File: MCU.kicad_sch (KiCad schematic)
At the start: 18 parts, among them U1 STM32L476RCTx, U3 LD1117S33TR, U5 nRF2401+ Module

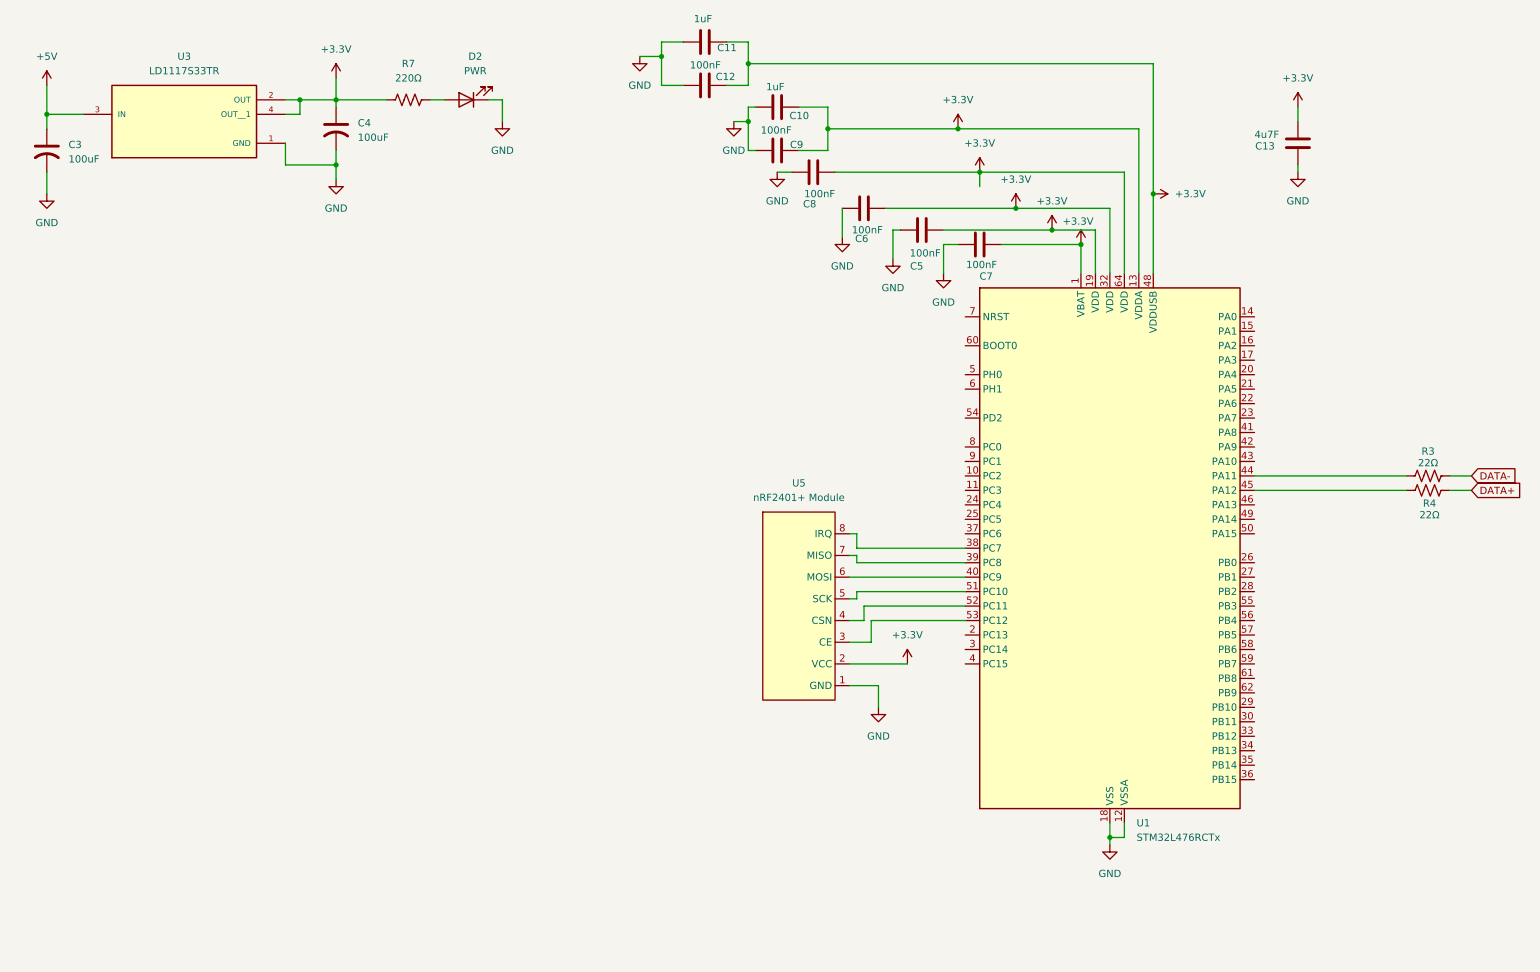
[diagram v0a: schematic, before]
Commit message: Everything is done except for the programming pins
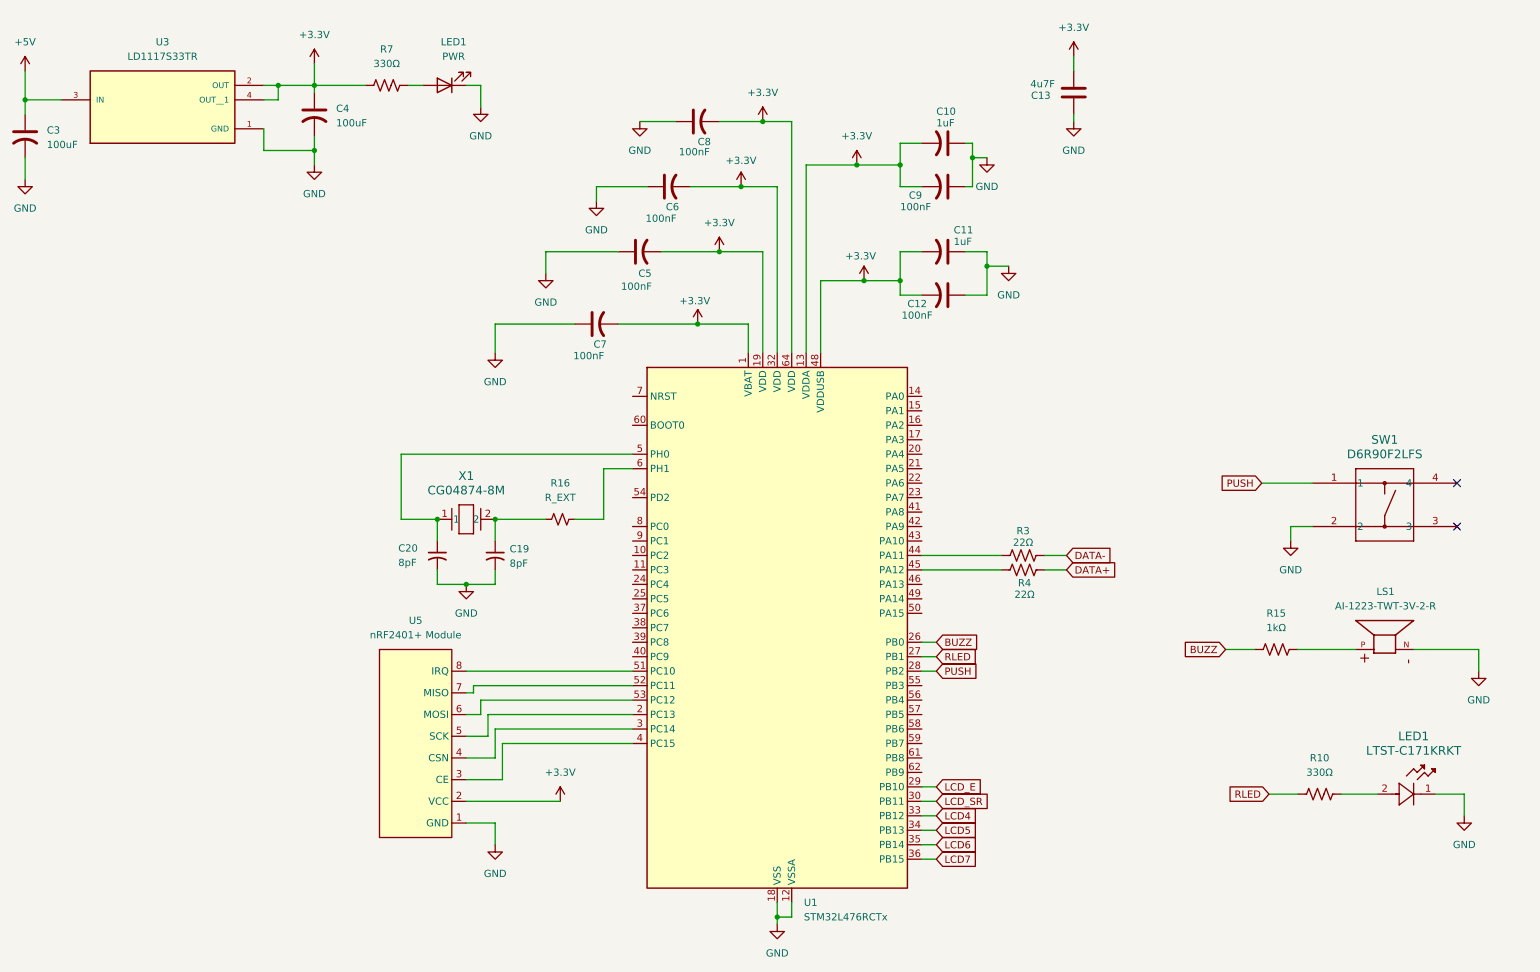
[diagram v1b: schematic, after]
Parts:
- added C19, C20: 8pF, symbol Device:C_Small_US
- added LED1: LTST-C171KRKT, LED_LTST-C171_LTO, symbol LTST-C171KRKT(red-LED):LTST-C171KRKT
- added LS1: AI-1223-TWT-3V-2-R, AI-1223-TWT-3V-2-R:XDCR_AI-1223-TWT-3V-2-R, symbol AI-1223-TWT-3V-2-R:AI-1223-TWT-3V-2-R
- added R10: 330Ω, symbol Device:R_US
- added R15: 1kΩ, symbol Device:R_US
- added R16: R_EXT, symbol Device:R_Small_US
- added SW1: D6R90F2LFS, D6R90_CNK, symbol D6R90_F2(push-button):D6R90F2LFS
- added X1: CG04874-8M, XTAL_CG04874_NDK, symbol CG04847-8M-XTAL:CG04874-8M
- C10, C11, C12, C5, C6, C7, C8, C9: symbol Device:C -> Device:C_US
- R7: value 220Ω -> 330Ω
- U5: footprint (none) -> nRF2401+_moduleBoard:HiLetgo-nRF2041+module
- renumbered D2 to LED1
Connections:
- net GND: now also C19.2, C20.2, LED1.1, LS1.N, SW1.2
- net at U1.2 (PC13): now also U5.5 (SCK)
- net BUZZ: now reaches U1.26 (PB0)
- net BUZZ: now also R15.2
- net RLED: now reaches U1.27 (PB1)
- net RLED: now also R10.1
- net PUSH: now reaches U1.28 (PB2)
- net PUSH: now also SW1.1
- net LCD_E: now reaches U1.29 (PB10)
- net at U1.3 (PC14): now also U5.4 (CSN)
- net LCD_SR: now reaches U1.30 (PB11)
- net LCD4: now reaches U1.33 (PB12)
- net LCD5: now reaches U1.34 (PB13)
- net LCD6: now reaches U1.35 (PB14)
- net LCD7: now reaches U1.36 (PB15)
- net at U1.38 (PC7): no longer U5.8 (IRQ)
- net at U1.39 (PC8): no longer U5.7 (MISO)
- net at U1.4 (PC15): now also U5.3 (CE)
- net at U1.40 (PC9): no longer U5.6 (MOSI)
- net at U1.5 (PH0): now also C20.1, X1.1
- net at U1.51 (PC10): now also U5.8 (IRQ); no longer U5.5 (SCK)
- net at U1.52 (PC11): now also U5.7 (MISO); no longer U5.4 (CSN)
- net at U1.53 (PC12): now also U5.6 (MOSI); no longer U5.3 (CE)
- net at U1.6 (PH1): now also R16.2
- new net: LS1.P, R15.1
- new net: C19.1, R16.1, X1.2
- new net: LED1.2, R10.2
- no-connect marks 0 -> 2
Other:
- moved on the sheet: C10, C11, C12, C13, C3, C4, C5, C6, C7, C8, C9, LED1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
